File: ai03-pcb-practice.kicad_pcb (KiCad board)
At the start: 2 copper layers, 74.6 x 38.1 mm, 24 parts, among them SW1 SW_Push, U1 ATmega32U4-A, Y1 16MHz

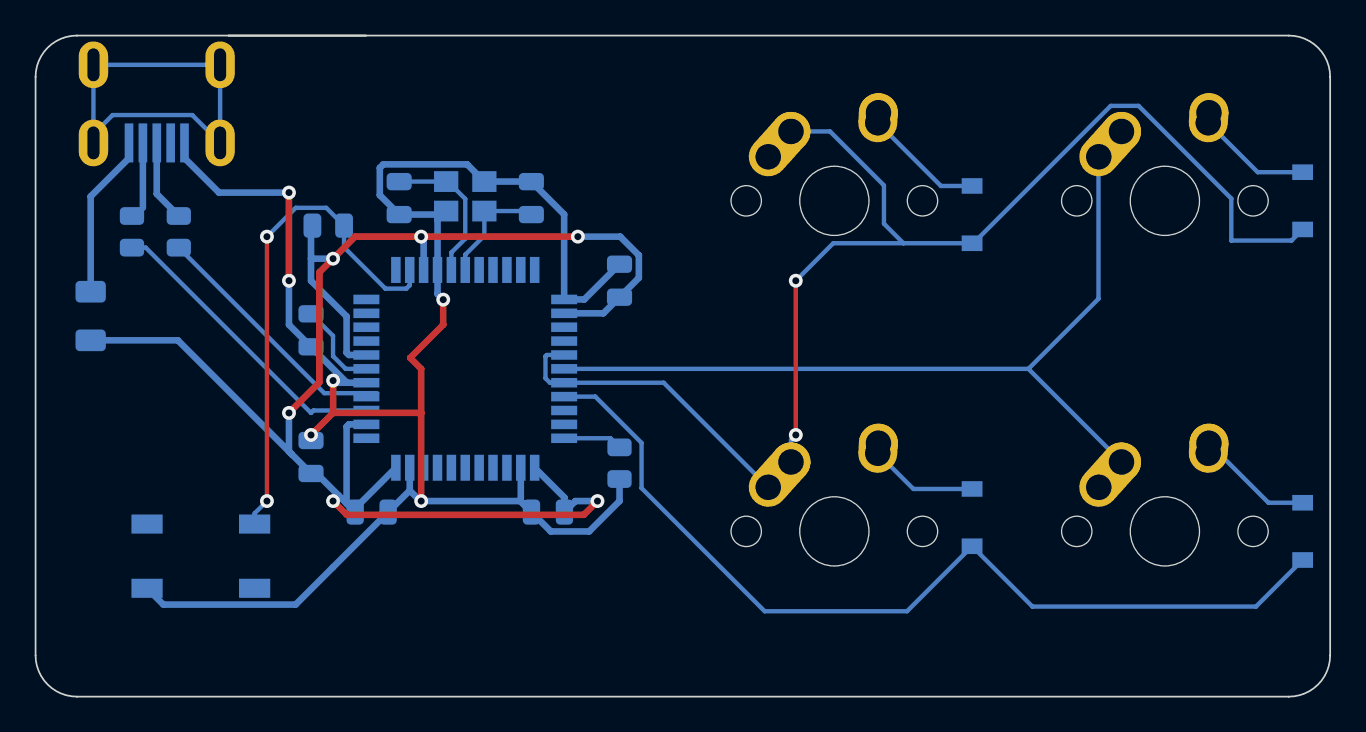
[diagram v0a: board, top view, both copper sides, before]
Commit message: Yup
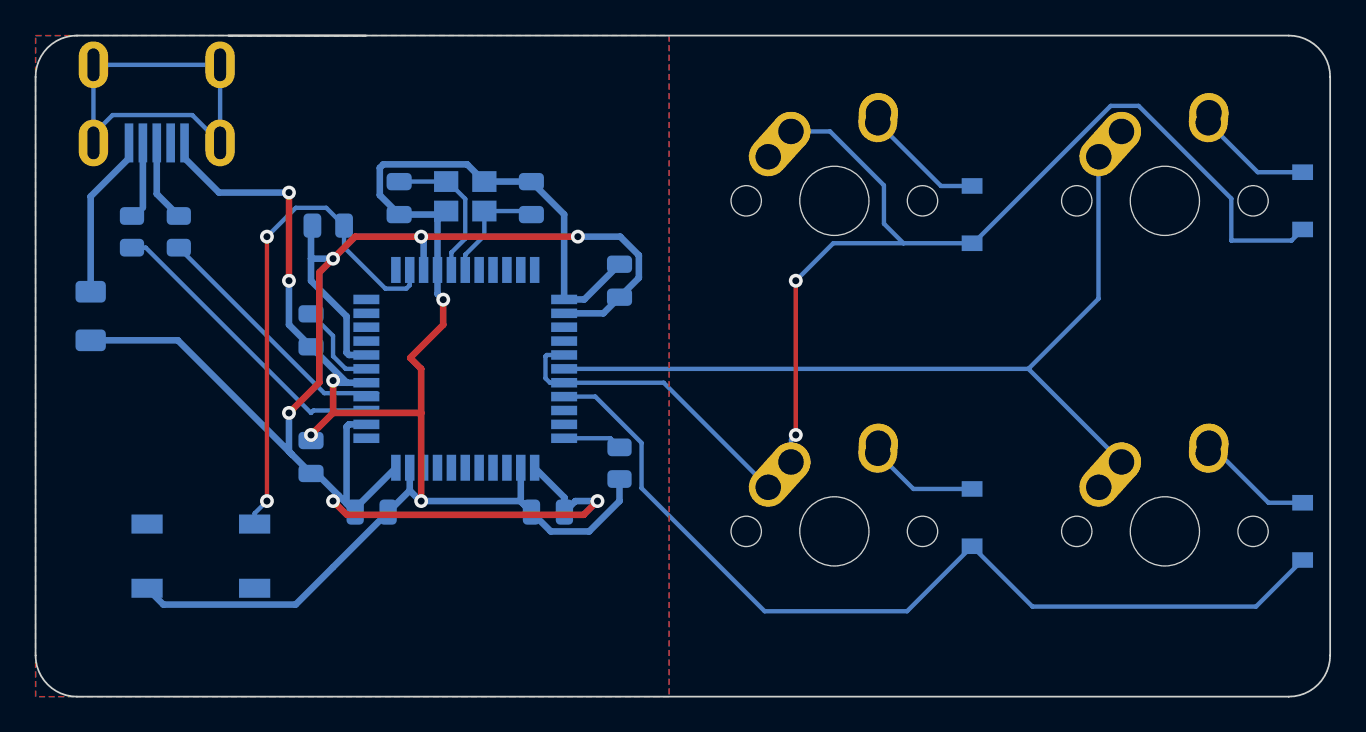
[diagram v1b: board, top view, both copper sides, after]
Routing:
- added copper zone on B.Cu, net GND
- added copper zone on F.Cu, net GND
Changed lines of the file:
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@@
   (segment (start 120.65 105.50625) (end 118.0625 105.50625) (width 0.254) (layer "B.Cu") (net 43))
   (segment (start 118.0625 105.50625) (end 115.2125 102.65625) (width 0.254) (layer "B.Cu") (net 43))
+  (zone (net 2) (net_name "GND") (layers F&B.Cu) (hatch edge 0.508)
+    (connect_pads (clearance 0.508))
+    (min_thickness 0.254) (filled_areas_thickness no)
+    (fill yes (thermal_gap 0.508) (thermal_bridge_width 0.508))
+    (polygon
+      (pts
+        (xy 84.1375 135.73125)
+        (xy 47.625 135.73125)
+        (xy 47.625 97.63125)
+        (xy 84.1375 97.63125)
+      )
+    )
+  )
 )
